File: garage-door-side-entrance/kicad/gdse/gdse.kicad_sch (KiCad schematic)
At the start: 3 parts, among them J1 Screw_Terminal_01x10

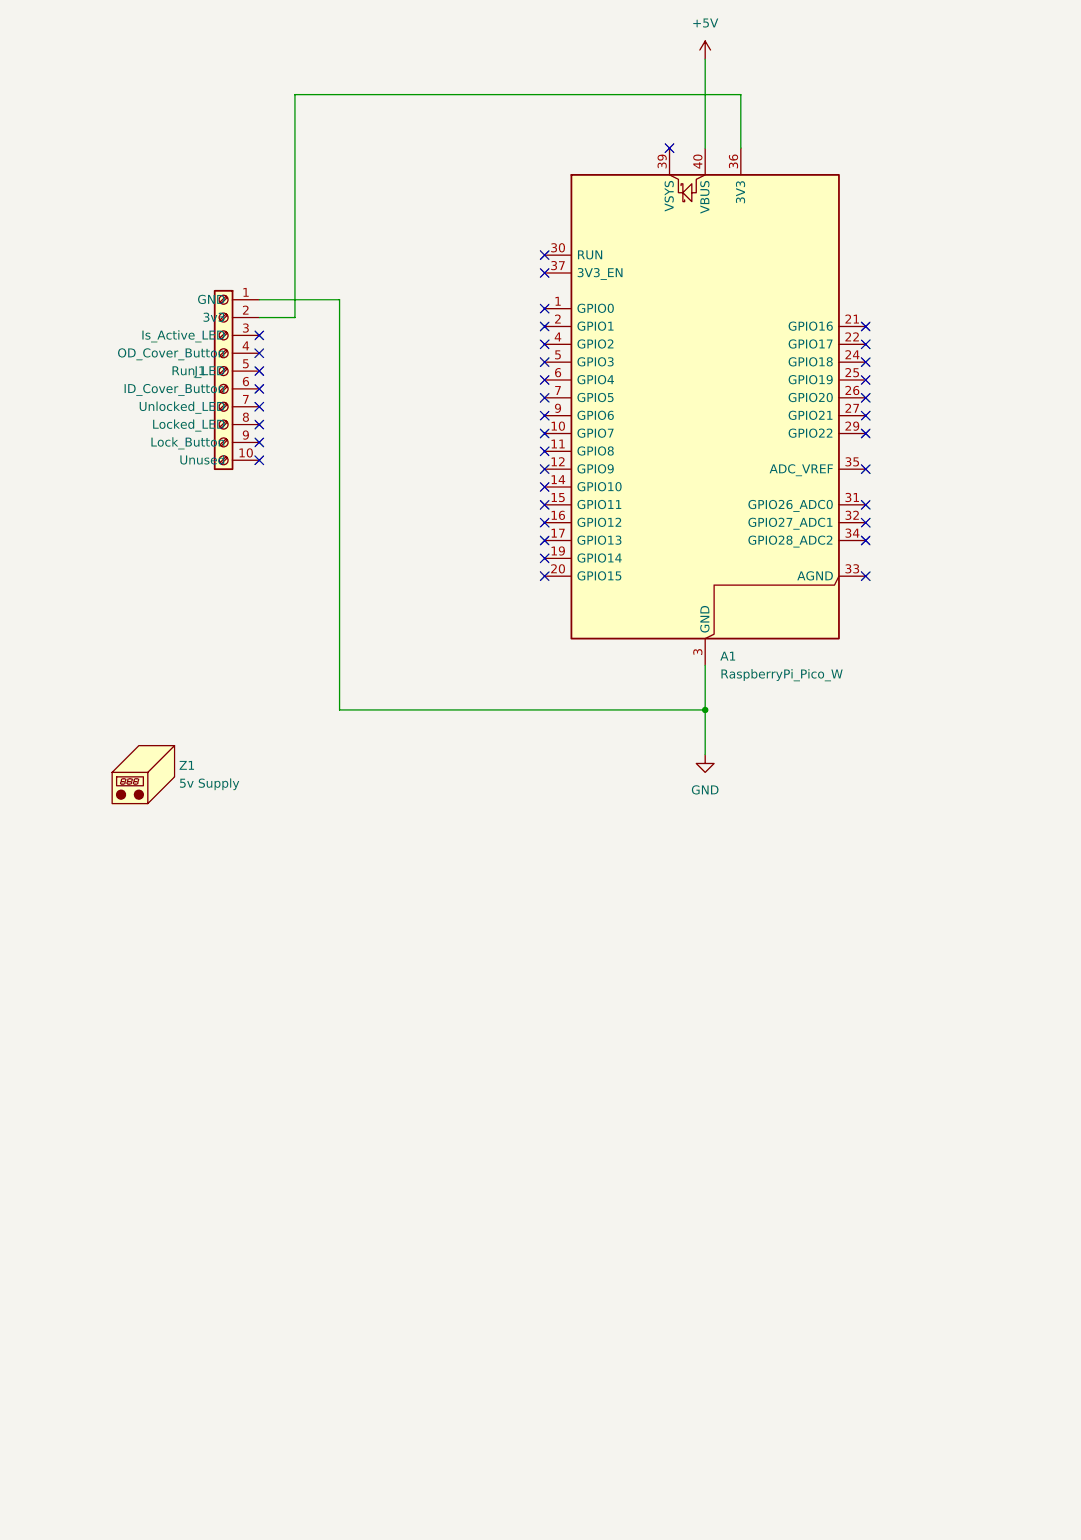
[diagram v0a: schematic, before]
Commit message: kicad work
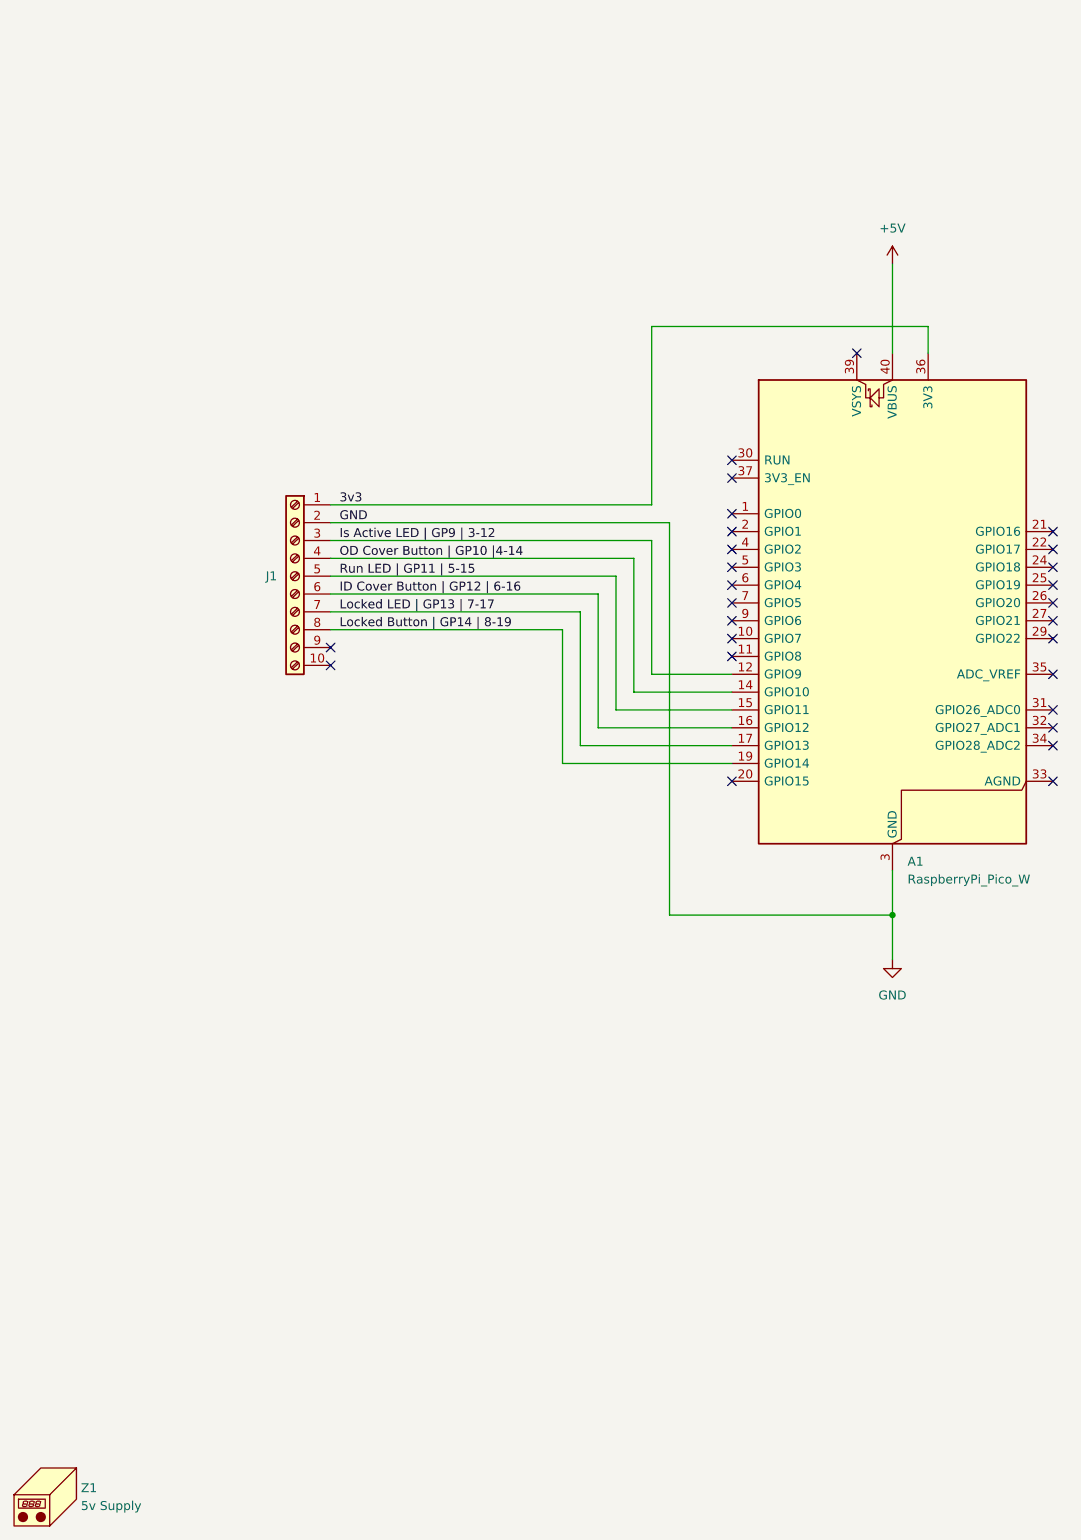
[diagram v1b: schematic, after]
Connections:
- net GND: now also J1.2 (Pin_2); no longer J1.1 (GND)
- net 3v3: now reaches A1.36 (3V3)
- net 3v3: now also J1.1 (Pin_1); no longer J1.2 (3v3)
- net Is Active LED | GP9 | 3-12: now reaches J1.3 (Pin_3)
- net Is Active LED | GP9 | 3-12: now also A1.12 (GPIO9)
- net OD Cover Button | GP10 |4-14: now reaches J1.4 (Pin_4)
- net OD Cover Button | GP10 |4-14: now also A1.14 (GPIO10)
- net Run LED | GP11 | 5-15: now reaches J1.5 (Pin_5)
- net Run LED | GP11 | 5-15: now also A1.15 (GPIO11)
- net ID Cover Button | GP12 | 6-16: now reaches J1.6 (Pin_6)
- net ID Cover Button | GP12 | 6-16: now also A1.16 (GPIO12)
- net Locked LED | GP13 | 7-17: now reaches J1.7 (Pin_7)
- net Locked LED | GP13 | 7-17: now also A1.17 (GPIO13)
- net Locked Button | GP14 | 8-19: now reaches J1.8 (Pin_8)
- net Locked Button | GP14 | 8-19: now also A1.19 (GPIO14)
- no-connect marks 39 -> 27
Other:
- moved on the sheet: A1, Z1
